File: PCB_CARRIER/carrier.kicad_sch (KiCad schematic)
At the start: 0 parts

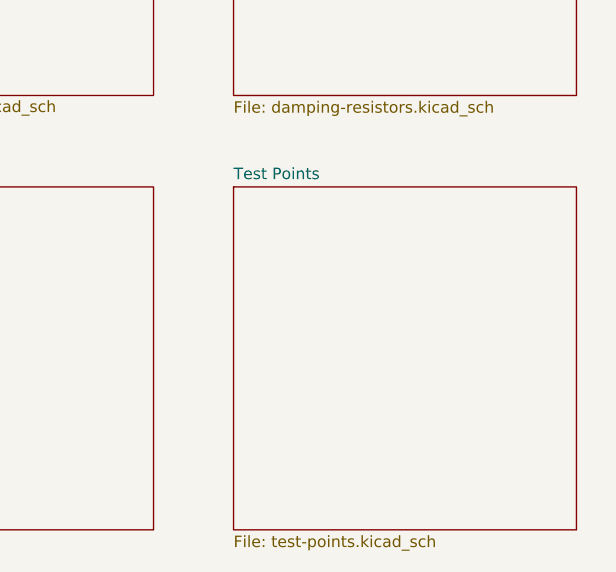
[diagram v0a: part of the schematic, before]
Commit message: finished adding test points
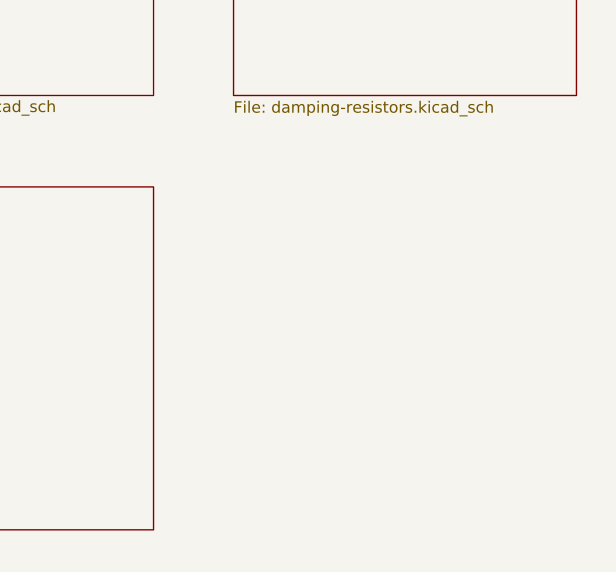
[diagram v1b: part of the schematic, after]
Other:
- removed sheet Test Points
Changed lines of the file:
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@@
-	)
-	(sheet
-		(at 71.12 121.92)
-		(size 38.1 38.1)
-		(exclude_from_sim no)
-		(in_bom yes)
-		(on_board yes)
-		(dnp no)
-		(fields_autoplaced yes)
-		(stroke
-			(width 0.1524)
-			(type solid)
-		)
-		(fill
-			(color 0 0 0 0.0000)
-		)
-		(property "Sheetname" "Test Points"
-			(at 71.12 121.2084 0)
-			(effects
-				(font
-					(size 1.27 1.27)
-				)
-				(justify left bottom)
-			)
-		)
-		(property "Sheetfile" "test-points.kicad_sch"
-			(at 71.12 160.6046 0)
-			(effects
-				(font
-					(size 1.27 1.27)
-				)
-				(justify left top)
-			)
-		)
-		(instances
-			(project "carrier"
-				(path "/f52509e6-8053-454c-b8e9-3e2670c5a5fe"
-					(page "7")
-				)
-			)
-		)
 	)
 	(sheet
